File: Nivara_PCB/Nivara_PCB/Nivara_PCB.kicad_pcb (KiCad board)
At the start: 4 copper layers, 98.8 x 81.2 mm, 160 parts, among them CN1 ANALOG_IN, CN2 RELAY, J1 AUXILIAR, K1 SRA-24VDC-CL, K2 SRA-24VDC-CL, P1 NPN_IN, P2 PNP_IN, P3 D_IN, P4 RUN/STOP, P5 NPN_OUT, P6 PNP_OUT, P7 RS485, P8 ANALOG_OUT., Q1 IRLML0040, Q2 AO3407A, Q3 IRLML0040, Q4 AO3407A, Q5 IRLML6402TRPBF-JSM, SW1 SKRPACE010, SW2 SKRPACE010, U1 2.54-2*2, U10 GP8201S-TC50-EW, U11 LK1802, U12 LTV-357T, U13 LTV-357T, U14 LTV-357T, U15 LTV-357T, U16 LTV-357T, U17 LTV-357T, U18 LTV-357T, U19 GP8303-TC50-EW, U2 FUENTE IN, U3 ESP32-S3-WROOM-1, U4 AP63200WU, U5 RSM3485ECHT_C2992406, U6 LTV-357T, U7 LTV-357T, U8 LTV-357T, U9 LTV-357T

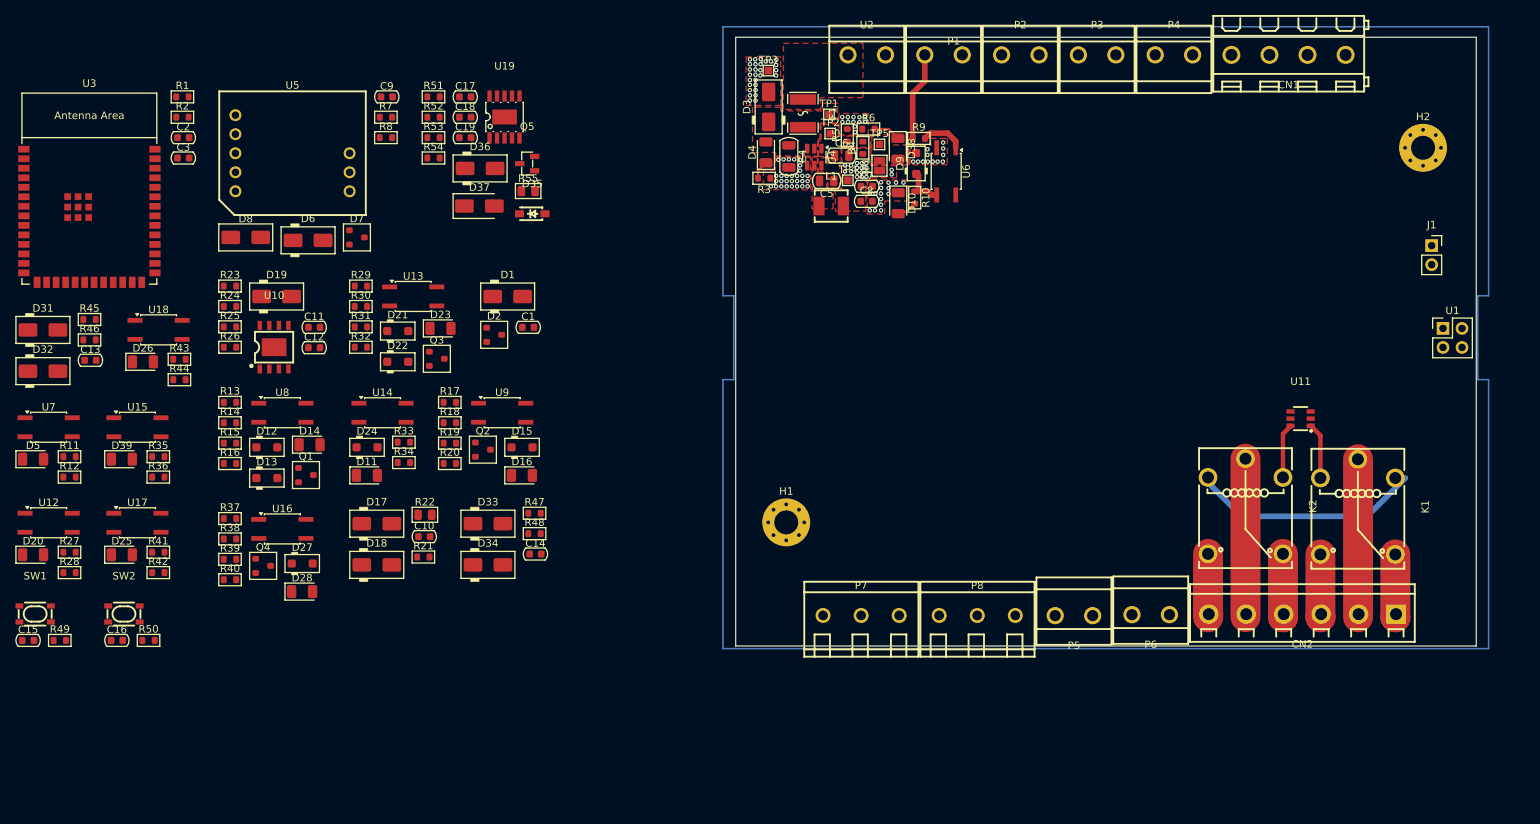
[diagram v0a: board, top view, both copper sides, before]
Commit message: Guardado los cambios con una sola fuente.
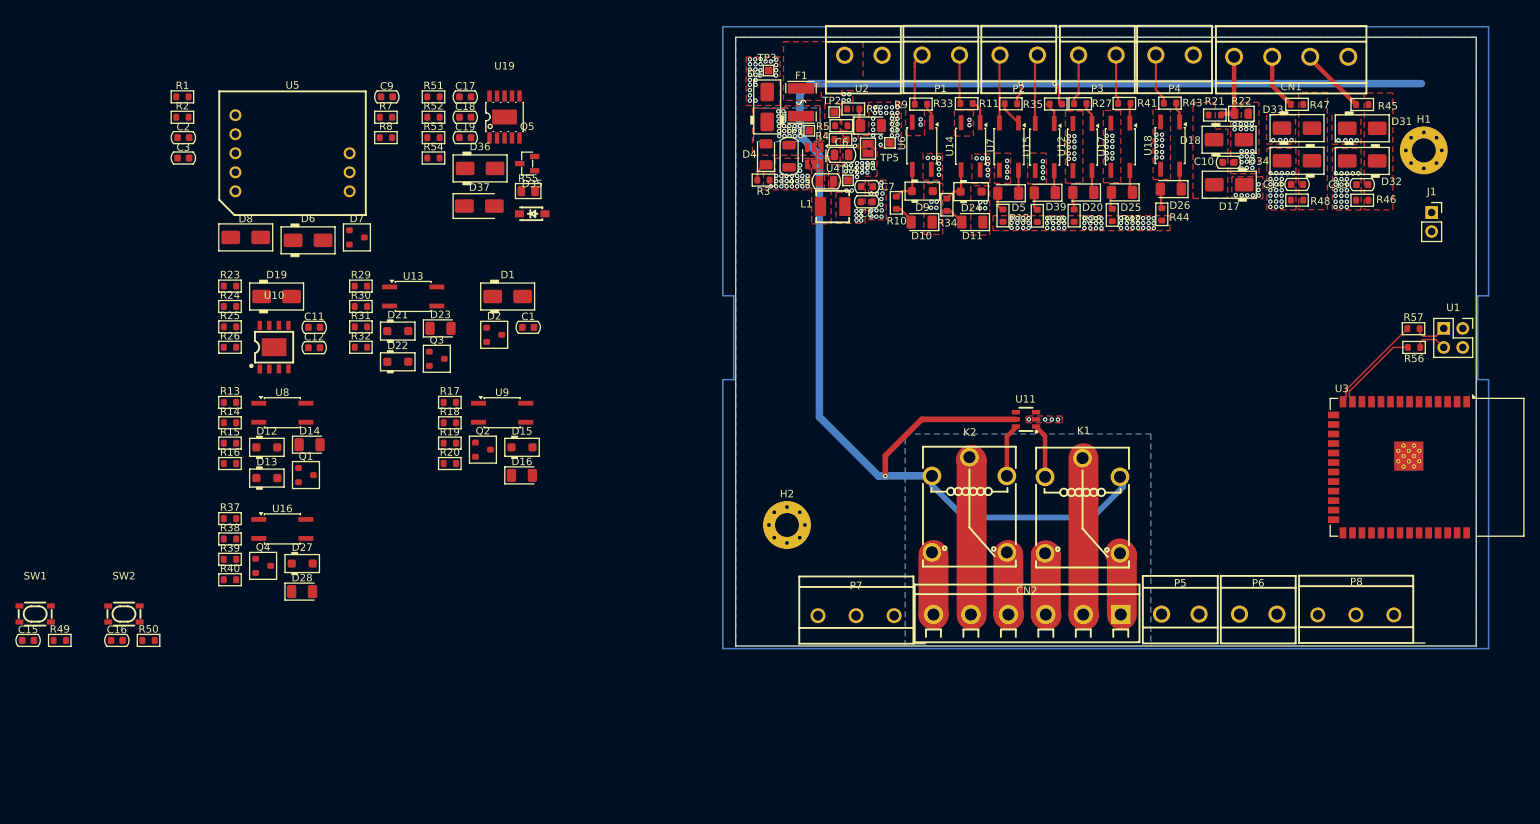
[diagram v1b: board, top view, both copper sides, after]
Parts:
- added R56: 33, PCM_Resistor_SMD_AKL:R_0603_1608Metric, F.Cu at (258.2, 82.8)
- added R57: 33, PCM_Resistor_SMD_AKL:R_0603_1608Metric, F.Cu at (258.1, 80.3)
- R1, R2: value 220 -> 33
- U1: footprint Connector_PinHeader_2.54mm:PinHeader_2x02_P2.54mm_Vertical -> Connector_PinSocket_2.54mm:PinSocket_2x02_P2.54mm_Vertical
- U3: footprint PCM_Espressif:ESP32-S3-WROOM-1 -> RF_Module:ESP32-S3-WROOM-1
- moved U3 181.8 mm to (260.0, 98.8), turned to -90 degrees
- moved D32 178.3 mm to (251.3, 57.9), turned to 180 degrees
- moved D31 178.1 mm to (251.3, 53.5)
- moved R45 172.3 mm to (251.3, 50.4), turned to 180 degrees
- moved C13 171.4 mm to (251.3, 61.1), turned to 180 degrees
- moved R46 170.9 mm to (251.3, 63.2)
- moved D20 148.3 mm to (214.1, 62.1), turned to 180 degrees
- moved R27 147.6 mm to (213.6, 50.3)
- moved U12 146.8 mm to (213.9, 56.1), turned to -90 degrees
- moved R28 142.3 mm to (212.8, 65.2), turned to 90 degrees
- moved R41 142.2 mm to (219.5, 50.2)
- moved D25 142.0 mm to (219.2, 62.1), turned to 180 degrees
- moved U17 140.5 mm to (219.0, 56.0), turned to -90 degrees
- moved D26 139.1 mm to (225.7, 61.7), turned to 180 degrees
- moved U18 137.2 mm to (225.6, 55.9), turned to -90 degrees
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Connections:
- net /NIVARA_BOARD/A_0-32_IN/A_OUT renamed /NIVARA_BOARD/A_0-32_IN/A_V_OUT
- D2 pad 1: /NIVARA_BOARD/USB_D+ -> /D+
- D2 pad 2: /NIVARA_BOARD/USB_D- -> /D-
- R47 pad 2: /NIVARA_BOARD/A_0-10_IN/A_V_IN -> /NIVARA_BOARD/A0_10_IN_1
- U1 pad 1: /NIVARA_BOARD/USB_D- -> GND
- U1 pad 2: GND -> /D-
- U1 pad 3: /NIVARA_BOARD/USB_D+ -> Net-(D1-A)
- U1 pad 4: Net-(D1-A) -> /D+
- U3 pad 13: /NIVARA_BOARD/USB_D- -> /NIVARA_BOARD/USB_D+
- U3 pad 14: /NIVARA_BOARD/USB_D+ -> /NIVARA_BOARD/USB_D-
- U3 pad 6: /NIVARA_BOARD/A_OUT -> /NIVARA_BOARD/A_0-10_IN/A_V_OUT
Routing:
- net VCC: track 30.8 -> 205.1 mm, vias 0 -> 24
- net /NIVARA_BOARD/USB_D-: track 0.00 -> 13.3 mm
- net /NIVARA_BOARD/USB_D+: track 0.00 -> 11.8 mm
- net /NIVARA_BOARD/PNP_IN_2: track 0.00 -> 9.90 mm
- net /NIVARA_BOARD/A4_20_IN_1: track 0.00 -> 9.50 mm
- net /NIVARA_BOARD/PNP_IN_1: track 0.00 -> 9.10 mm
- net /NIVARA_BOARD/A0_32_IN_1: track 0.00 -> 8.91 mm
- net /NIVARA_BOARD/A0_10_IN_1: track 0.00 -> 7.39 mm
- net /NIVARA_BOARD/RUN/STOP: track 0.00 -> 6.87 mm
- net /NIVARA_BOARD/D_IN_1: track 0.00 -> 6.75 mm
- net /NIVARA_BOARD/D_IN_2: track 0.00 -> 6.58 mm
- net /NIVARA_BOARD/NPN_IN_2: track 0.00 -> 6.53 mm
- net /NIVARA_BOARD/NPN_IN_2/NPN_OUT: track 0.00 -> 5.30 mm
- net /NIVARA_BOARD/NPN_IN_1: track 11.8 -> 6.97 mm
- net /D+: track 0.00 -> 4.39 mm
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- added copper zone on In2.Cu, net +3.3V
- added copper zone on F.Cu, net /NIVARA_BOARD/4-20mA_IN/ESP_4-20_IN
- added copper zone on F.Cu, net /NIVARA_BOARD/A_0-10_IN/A_V_OUT
- added copper zone on F.Cu, net /NIVARA_BOARD/A_0-32_IN/A_V_OUT
- added copper zone on B.Cu, net GND
- added copper zone on B.Cu, net VCC

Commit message: Saved changes to Nivara PCB files
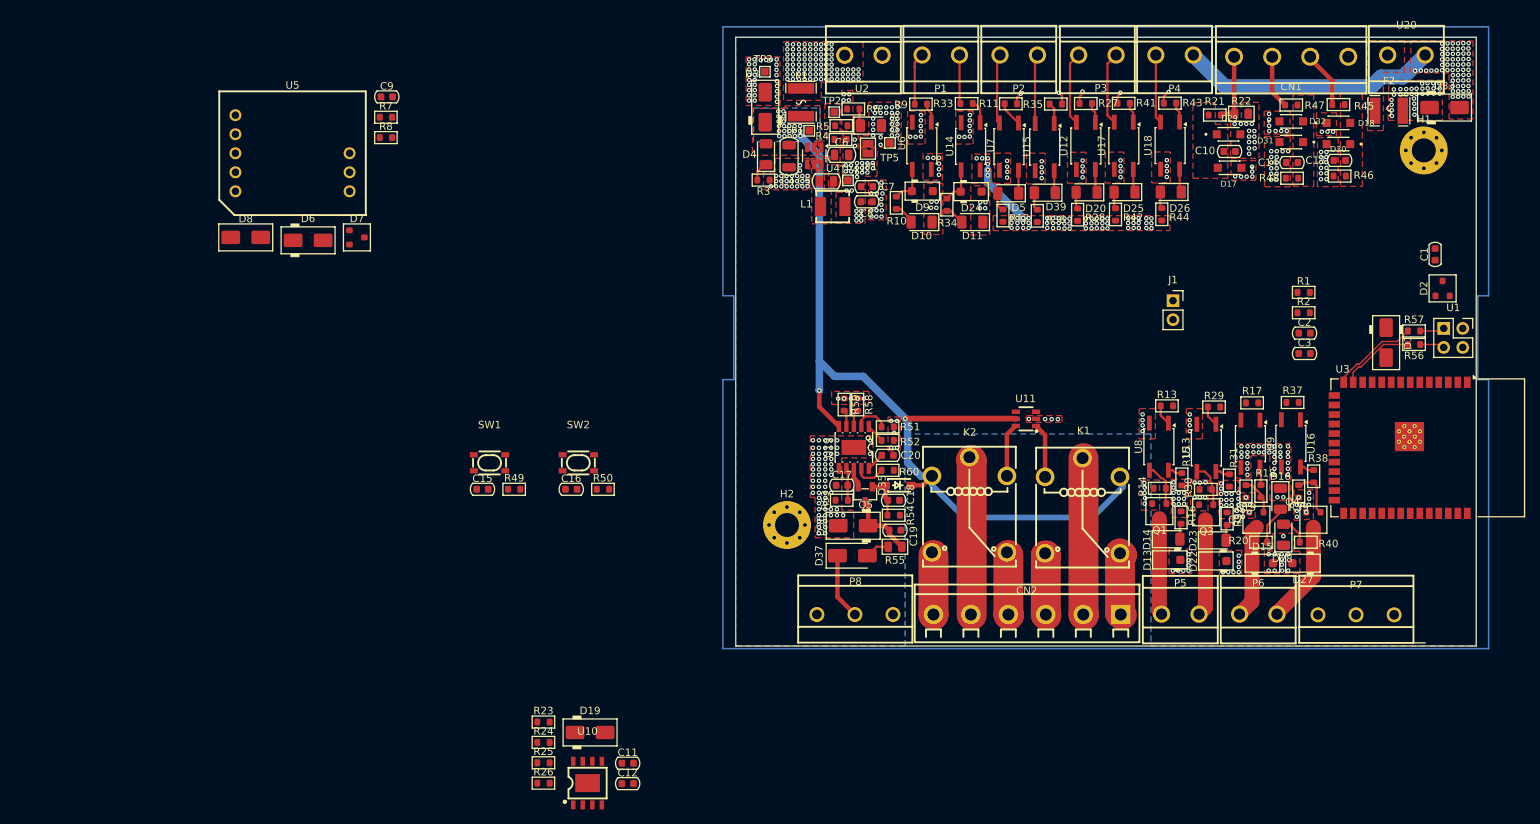
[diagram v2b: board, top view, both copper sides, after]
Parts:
- removed D12, D21: PMEG4010CEH, PCM_Diode_SMD_AKL:D_SOD-123F
- removed D34: SMAJ5.0A, PCM_Diode_SMD_AKL:D_SMA
- added C20: 1uF, PCM_Capacitor_SMD_AKL:C_0603_1608Metric, F.Cu at (187.9, 97.2)
- added D29: SMF5.0A, SMF5.0A:SODFL3718X102N, F.Cu at (233.4, 54.3)
- added D30: SMF5.0A, SMF5.0A:SODFL3718X102N, F.Cu at (248.1, 55.7)
- added F2: BSMD1812-150-33V, EasyEDA:F1812, F.Cu at (254.8, 51.2)
- added R58: 22k, PCM_Resistor_SMD_AKL:R_0603_1608Metric, F.Cu at (183.9, 90.4)
- added R59: 22k, PCM_Resistor_SMD_AKL:R_0603_1608Metric, F.Cu at (182.1, 90.4)
- added R60: 22k, PCM_Resistor_SMD_AKL:R_0603_1608Metric, F.Cu at (187.9, 99.2)
- added U20: FUENTE EX, EasyEDA:CONN-TH_XY126V-5.0-2P, F.Cu at (257.2, 43.8)
- D17, D18, D31, D32: value SMAJ5.0A -> SMF5.0A; footprint PCM_Diode_SMD_AKL:D_SMA -> SMF5.0A:SODFL3718X102N
- D33: value SMAJ5.0A -> SMAJ33A
- R15, R31: value 20k -> 30k
- moved C2 151.9 mm to (243.6, 80.9)
- moved C3 151.9 mm to (243.6, 83.6)
- moved R1 151.9 mm to (243.5, 75.4)
- moved R2 151.9 mm to (243.5, 78.2)
- moved R38 144.9 mm to (244.8, 100.0), turned to 90 degrees
- moved R40 143.7 mm to (243.8, 108.8), turned to 180 degrees
- moved R39 142.9 mm to (242.8, 102.0), turned to 90 degrees
- moved R37 142.7 mm to (242.0, 90.2)
- moved Q4 140.3 mm to (244.8, 105.8), turned to -90 degrees
- moved U16 135.1 mm to (241.8, 95.6), turned to -90 degrees
- moved D27 133.6 mm to (243.4, 111.6), turned to 180 degrees
- moved D28 131.2 mm to (240.8, 107.8), turned to 90 degrees
- moved R16 127.1 mm to (227.1, 105.5), turned to -90 degrees
- moved R15 127.1 mm to (227.2, 100.4), turned to 90 degrees
- moved D2 126.7 mm to (262.0, 74.9), turned to 90 degrees
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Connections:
- D13 pad 1: VCC -> VDD
- D13 pad 2: /NIVARA_BOARD/NPN_OUT_1/NPN_OUT -> /NIVARA_BOARD/NPN_OUT_1
- D14 pad 1: /NIVARA_BOARD/NPN_OUT_1/NPN_OUT -> /NIVARA_BOARD/NPN_OUT_1
- D15 pad 2: GND -> Earth
- D16 pad 1: GND -> Earth
- D22 pad 1: VCC -> VDD
- D22 pad 2: /NIVARA_BOARD/NPN_OUT_2/NPN_OUT -> /NIVARA_BOARD/NPN_OUT_2
- D23 pad 1: /NIVARA_BOARD/NPN_OUT_2/NPN_OUT -> /NIVARA_BOARD/NPN_OUT_2
- D27 pad 2: GND -> Earth
- D28 pad 1: GND -> Earth
- D33 pad 1: +3.3V -> VDD
- D33 pad 2: /NIVARA_BOARD/A_0-10_IN/A_V_OUT -> Earth
- P4 pad 2: GND -> Earth
- Q1 pad 2: GND -> Earth
- Q1 pad 3: /NIVARA_BOARD/NPN_OUT_1/NPN_OUT -> /NIVARA_BOARD/NPN_OUT_1
- Q2 pad 2: VCC -> VDD
- Q3 pad 2: GND -> Earth
- Q3 pad 3: /NIVARA_BOARD/NPN_OUT_2/NPN_OUT -> /NIVARA_BOARD/NPN_OUT_2
- Q4 pad 2: VCC -> VDD
- R11 pad 1: VCC -> VDD
- R13 pad 1: /NIVARA_BOARD/NPN_OUT_1 -> /NIVARA_BOARD/NPN_OUT_1/NPN_IN
- R14 pad 2: GND -> Earth
- R15 pad 1: VCC -> VDD
- R16 pad 1: VCC -> VDD
- R19 pad 1: VCC -> VDD
- R27 pad 1: /NIVARA_BOARD/D_IN_1 -> VDD
- R29 pad 1: /NIVARA_BOARD/NPN_OUT_2 -> /NIVARA_BOARD/NPN_OUT_2/NPN_IN
- R30 pad 2: GND -> Earth
- R31 pad 1: VCC -> VDD
- R32 pad 1: VCC -> VDD
- R35 pad 1: VCC -> VDD
- R39 pad 1: VCC -> VDD
- R41 pad 1: /NIVARA_BOARD/D_IN_2 -> VDD
- R43 pad 1: /NIVARA_BOARD/RUN/STOP -> VDD
- U12 pad 2: GND -> /NIVARA_BOARD/D_IN_1
- U14 pad 2: GND -> Earth
- U16 pad 3: GND -> Earth
- U17 pad 2: GND -> /NIVARA_BOARD/D_IN_2
- U18 pad 2: GND -> /NIVARA_BOARD/RUN/STOP
- U19 pad 10: unconnected-(U19-V5V-Pad10) -> Net-(U19-V5V)
- U19 pad 11: unconnected-(U19-EP-Pad11) -> GND
- U19 pad 3: unconnected-(U19-A0-Pad3) -> Net-(U19-A0)
- U19 pad 4: unconnected-(U19-A1-Pad4) -> Net-(U19-A1)
- U19 pad 9: unconnected-(U19-A2-Pad9) -> Net-(U19-A2)
- U3 pad 34: /NIVARA_BOARD/NPN_OUT_1/NPN_OUT -> /NIVARA_BOARD/NPN_OUT_1/NPN_IN
- U3 pad 35: /NIVARA_BOARD/NPN_OUT_2/NPN_OUT -> /NIVARA_BOARD/NPN_OUT_2/NPN_IN
- U6 pad 2: GND -> Earth
- U9 pad 3: GND -> Earth
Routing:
- net VCC: track 205.1 -> 116.2 mm, vias 24 -> 23
- net Earth: track 0.00 -> 34.5 mm, vias 0 -> 131
- net /NIVARA_BOARD/PNP_OUT_2: track 0.00 -> 13.6 mm
- net /NIVARA_BOARD/NPN_OUT_2: track 0.00 -> 13.0 mm
- net /NIVARA_BOARD/NPN_OUT_1: track 0.00 -> 12.9 mm
- net /NIVARA_BOARD/PNP_OUT_1: track 0.00 -> 12.5 mm
- net Net-(D36-K): track 0.00 -> 11.2 mm
- net /NIVARA_BOARD/I_OUT: track 0.00 -> 8.82 mm
- net +3.3V: track 0.00 -> 8.40 mm, vias 108 -> 114
- net VDD: track 0.00 -> 8.36 mm, vias 0 -> 91
- net Net-(Q4-G): track 0.00 -> 6.14 mm
- net Net-(Q3-G): track 0.00 -> 6.07 mm
- net Net-(D35-A): track 0.00 -> 5.99 mm
- net Net-(Q1-G): track 0.00 -> 5.63 mm
- net Net-(D16-A): track 0.00 -> 5.14 mm
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- added copper zone on F.Cu, net Earth
- added copper zone on In1.Cu, net Earth
- added copper zone on F.Cu, net Net-(F2-Pad1)
- added copper zone on B.Cu, net VDD
- added copper zone on F.Cu, net VDD
- removed copper zone on B.Cu, net GND
